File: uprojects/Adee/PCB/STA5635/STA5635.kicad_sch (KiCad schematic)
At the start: 1 part, among them U1 STA5635A

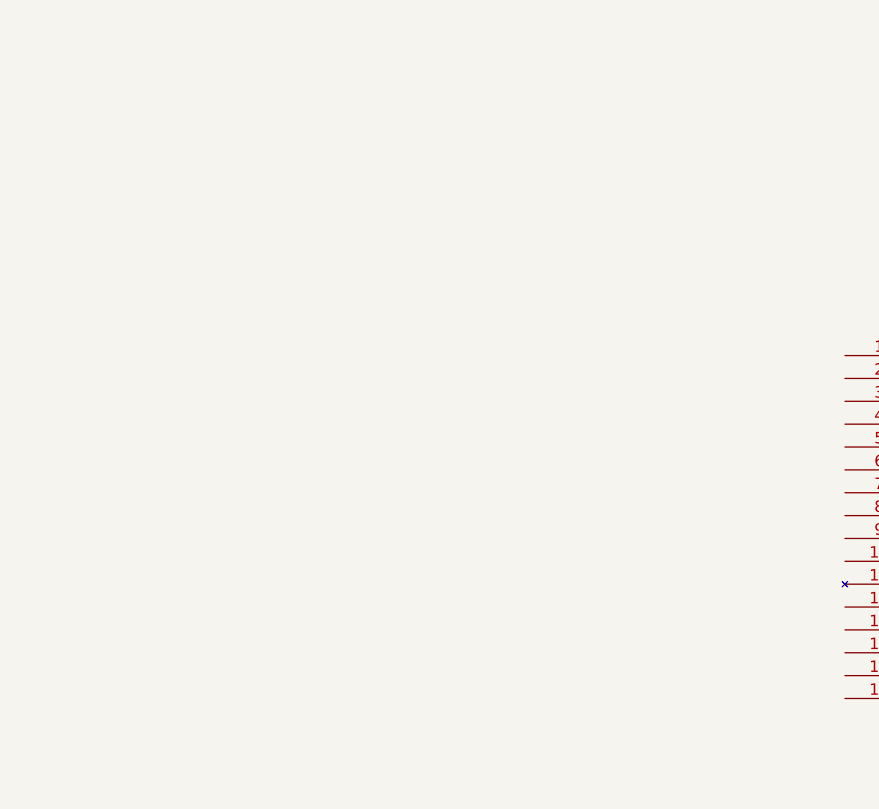
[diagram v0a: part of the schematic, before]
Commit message: 1-august 24
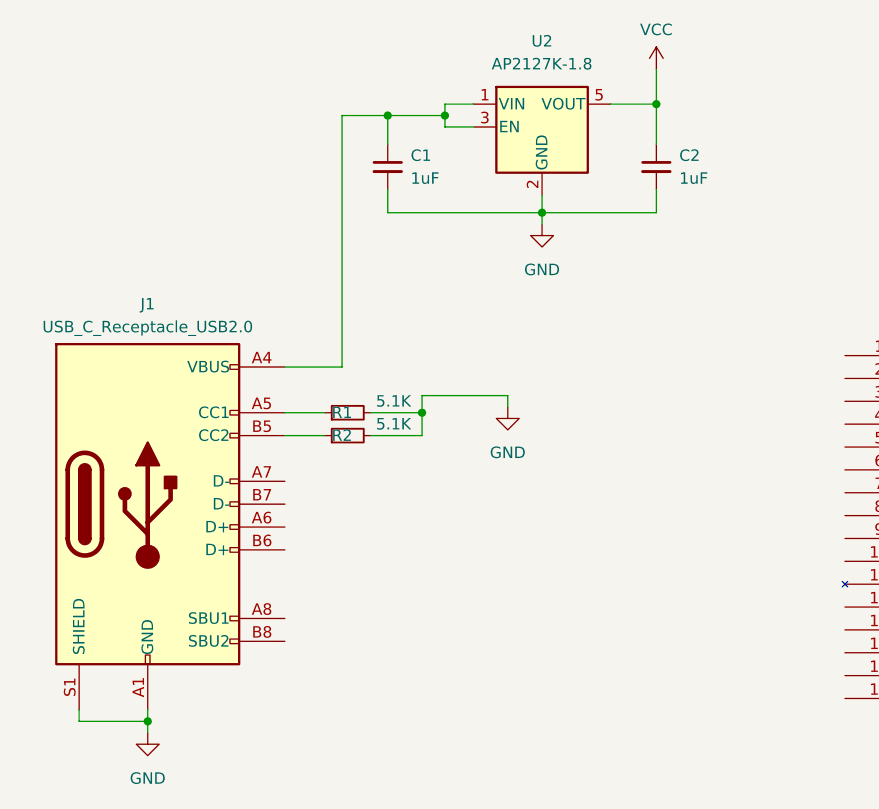
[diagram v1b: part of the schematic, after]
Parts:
- added C1, C2: 1uF, symbol Device:C_Small
- added J1: USB_C_Receptacle_USB2.0, symbol Connector:USB_C_Receptacle_USB2.0
- added R1, R2: 5.1K, symbol Device:R_Small
- added U2: AP2127K-1.8, Package_TO_SOT_SMD:SOT-23-5, symbol Regulator_Linear:AP2127K-1.8
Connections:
- new net: J1.A5 (CC1), R1.1
- new net: C1.1, J1.A4 (VBUS), J1.A9 (VBUS), J1.B4 (VBUS), J1.B9 (VBUS), U2.1 (VIN), U2.3 (EN)
- new net: J1.B5 (CC2), R2.1
- new net GND: C1.2, C2.2, J1.A1 (GND), J1.A12 (GND), J1.B1 (GND), J1.B12 (GND), J1.S1 (SHIELD), R1.2, R2.2, U2.2 (GND)
- new net VCC: C2.1, U2.5 (VOUT)

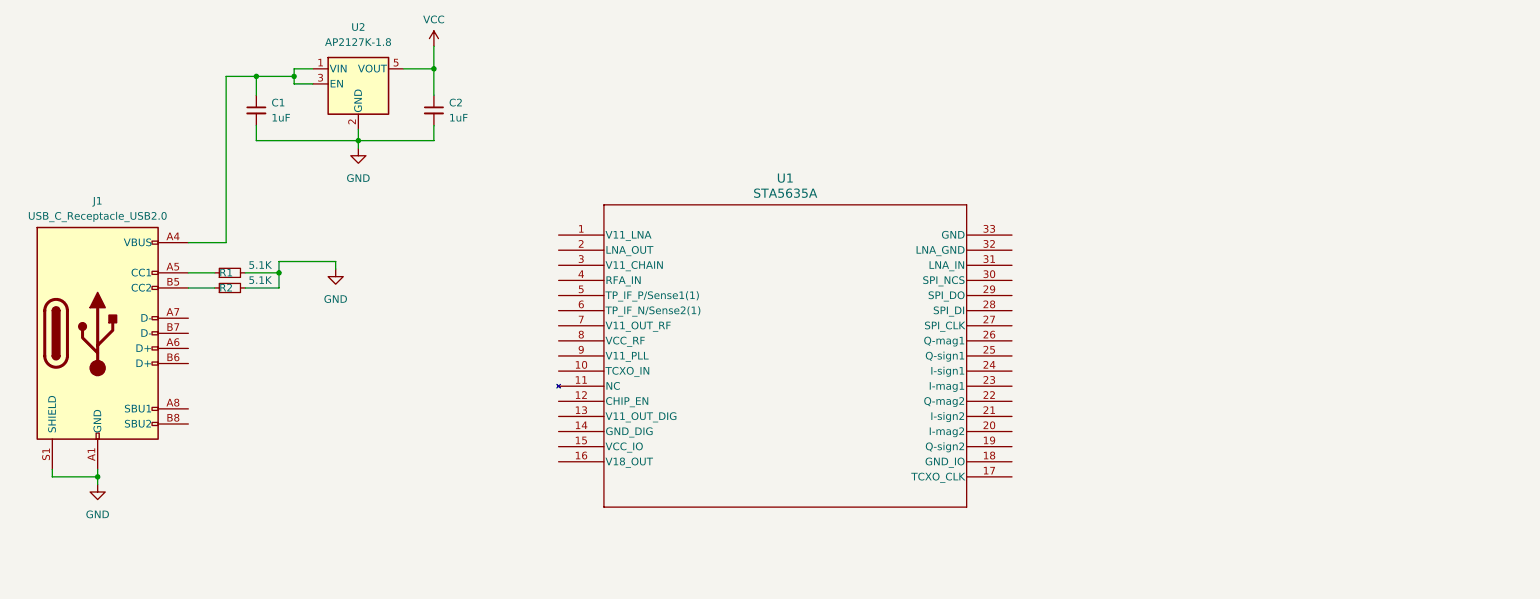
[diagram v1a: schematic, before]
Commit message: 3-august 24
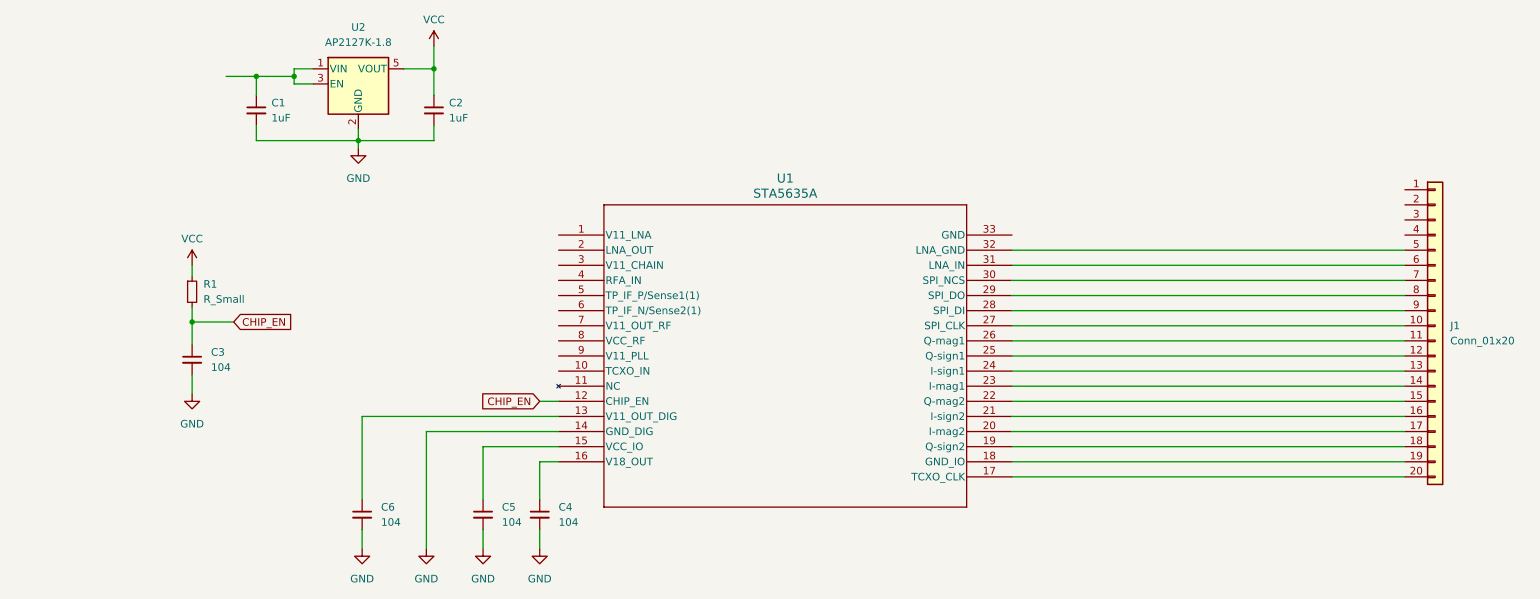
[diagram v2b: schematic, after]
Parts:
- removed J1: USB_C_Receptacle_USB2.0, symbol Connector:USB_C_Receptacle_USB2.0
- removed R2: 5.1K, symbol Device:R_Small
- added C3, C4, C5, C6: 104, Capacitor_SMD:C_1206_3216Metric, symbol Device:C_Small
- added J1: Conn_01x20, Connector_PinHeader_2.54mm:PinHeader_1x20_P2.54mm_Vertical, symbol Connector_Generic:Conn_01x20
- C1, C2: footprint (none) -> Capacitor_SMD:C_1206_3216Metric
- R1: value 5.1K -> R_Small
- U1: footprint VFQPN_A5635A_STM -> VFQPN_A5635A_STM:VFQPN_A5635A_STM
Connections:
- net GND: now also U1.14 (GND_DIG), C3.2, C4.2, C5.2, C6.2; no longer R1.2
- net VCC: now also R1.1
- net CHIP_EN: now reaches U1.12 (CHIP_EN)
- net CHIP_EN: now also R1.2, C3.1
- net at U1.13 (V11_OUT_DIG): now also C6.1
- net at U1.15 (VCC_IO): now also C5.1
- net at U1.16 (V18_OUT): now also C4.1
- net at U1.17 (TCXO_CLK): now also J1.20 (Pin_20)
- net at U1.18 (GND_IO): now also J1.19 (Pin_19)
- net at U1.19 (Q-sign2): now also J1.18 (Pin_18)
- net at U1.20 (I-mag2): now also J1.17 (Pin_17)
- net at U1.21 (I-sign2): now also J1.16 (Pin_16)
- net at U1.22 (Q-mag2): now also J1.15 (Pin_15)
- net at U1.23 (I-mag1): now also J1.14 (Pin_14)
- net at U1.24 (I-sign1): now also J1.13 (Pin_13)
- net at U1.25 (Q-sign1): now also J1.12 (Pin_12)
- net at U1.26 (Q-mag1): now also J1.11 (Pin_11)
- net at U1.27 (SPI_CLK): now also J1.10 (Pin_10)
- net at U1.28 (SPI_DI): now also J1.9 (Pin_9)
- net at U1.29 (SPI_DO): now also J1.8 (Pin_8)
- net at U1.30 (SPI_NCS): now also J1.7 (Pin_7)
- net at U1.31 (LNA_IN): now also J1.6 (Pin_6)
- net at U1.32 (LNA_GND): now also J1.5 (Pin_5)
